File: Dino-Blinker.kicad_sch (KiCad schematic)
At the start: 26 parts, among them IC1 M74HC4060YRM13TR, J1 Conn_01x02_Pin

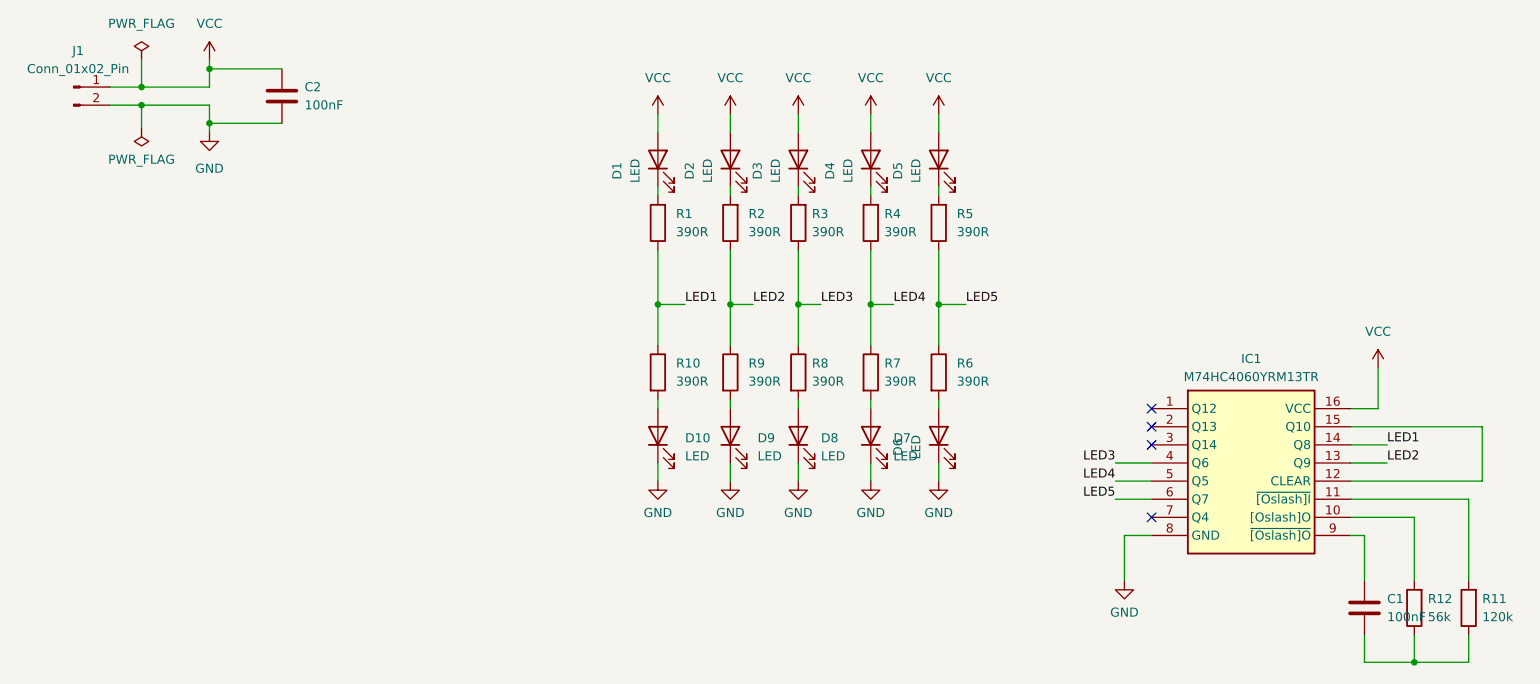
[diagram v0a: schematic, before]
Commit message: run kibot
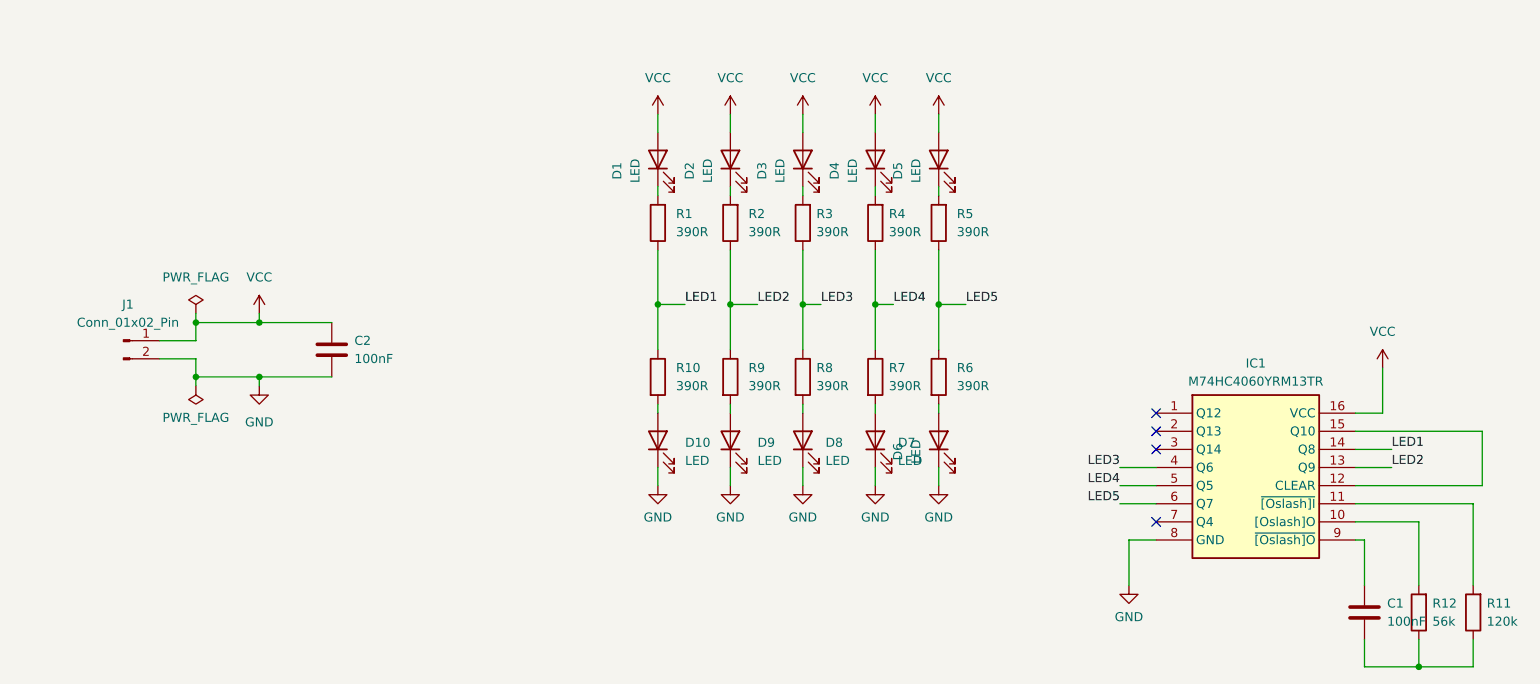
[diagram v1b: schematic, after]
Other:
- moved on the sheet: C1, C2, D10, D3, D4, D6, D7, D8, D9, IC1, J1, R10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
